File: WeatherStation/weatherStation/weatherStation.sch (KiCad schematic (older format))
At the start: 34 parts, among them J1 RJ12, J3 AVR-ISP-6, J4 USB_B_Micro, SW1 SW_Push, U1 ATmega328P-AU, U2 ATtiny45V-10PU, U3 BME280, U4 FDW254p, U5 FT230XS, U6 MB85RC64, U7 DS3231_Breakout, Y1 Crystal

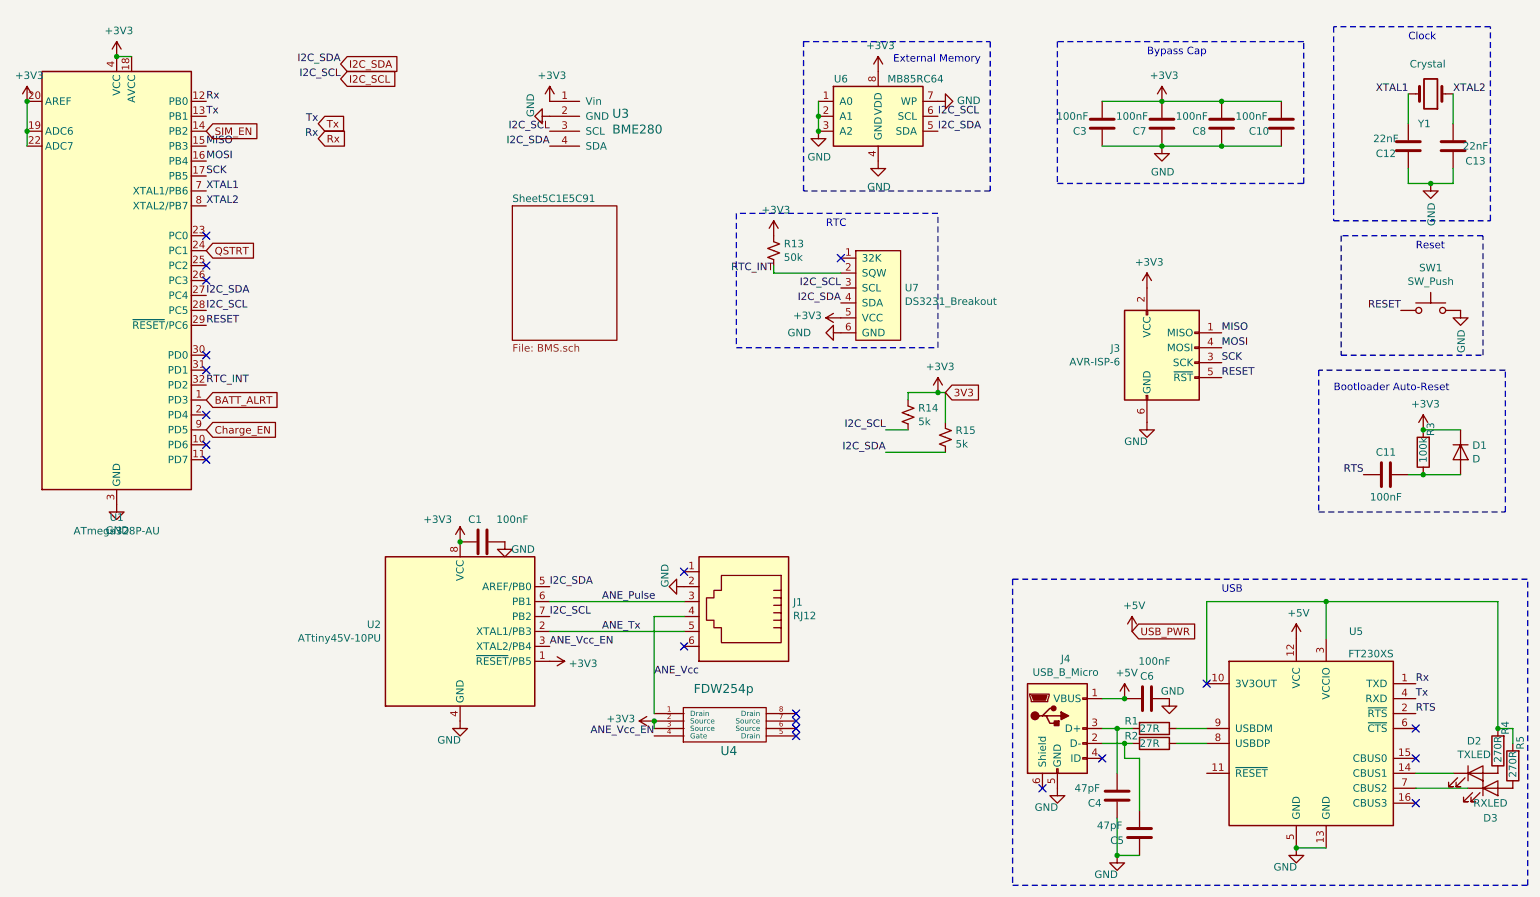
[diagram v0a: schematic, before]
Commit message: commit before more
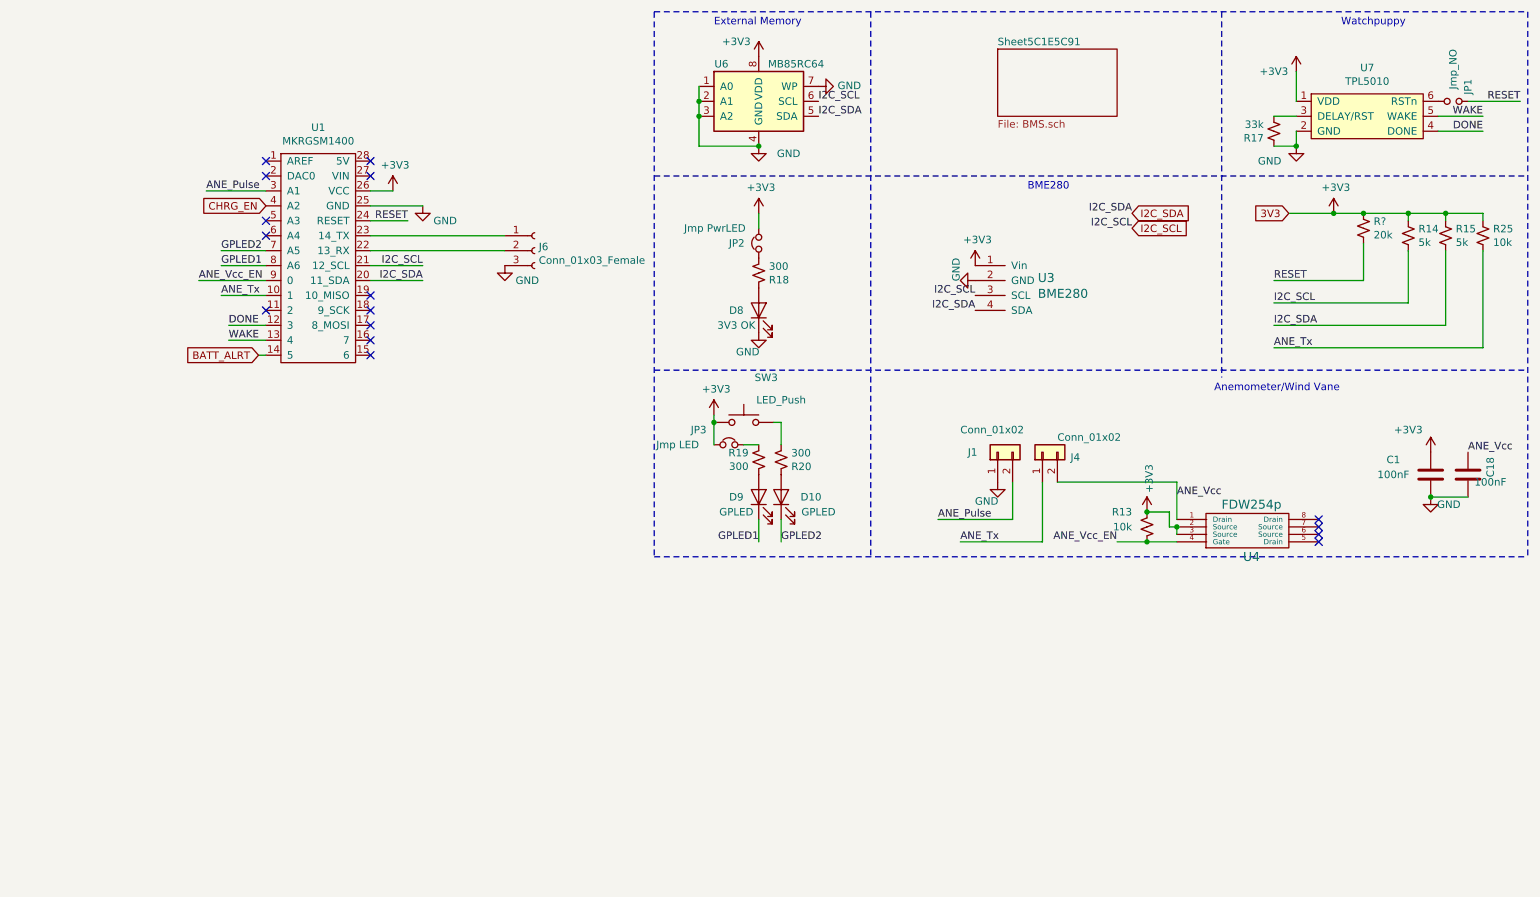
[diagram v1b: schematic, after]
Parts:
- removed C10, C11, C3, C6, C7, C8: 100nF, Capacitor_SMD:C_0805_2012Metric, symbol Device:C
- removed C12, C13: 22nF, Capacitor_SMD:C_0805_2012Metric, symbol Device:C
- removed C4, C5: 47pF, Capacitor_SMD:C_0805_2012Metric, symbol Device:C
- removed D1: D, Diode_SMD:D_SOD-323, symbol Device:D
- removed D2: TXLED, LED_SMD:LED_0805_2012Metric, symbol Device:LED
- removed D3: RXLED, LED_SMD:LED_0805_2012Metric, symbol Device:LED
- removed J1: RJ12, Connector_RJ:RJ12_Amphenol_54601, symbol Connector:RJ12
- removed J3: AVR-ISP-6, Connector_PinHeader_2.54mm:PinHeader_2x03_P2.54mm_Vertical, symbol Connector:AVR-ISP-6
- removed J4: USB_B_Micro, Connector_USB:USB_Micro-B_Amphenol_10103594-0001LF_Horizontal, symbol Connector:USB_B_Micro
- removed R1, R2: 27R, Resistor_SMD:R_0603_1608Metric_Pad1.05x0.95mm_HandSolder, symbol Device:R
- removed R3: 100k, Resistor_SMD:R_0603_1608Metric_Pad1.05x0.95mm_HandSolder, symbol Device:R
- removed R4, R5: 270R, Resistor_SMD:R_0805_2012Metric, symbol Device:R
- removed SW1: SW_Push, EbayParts:Tact_SMD_Switch, symbol Switch:SW_Push
- removed U1: ATmega328P-AU, Package_QFP:TQFP-32_7x7mm_P0.8mm, symbol MCU_Microchip_ATmega:ATmega328P-AU
- removed U2: ATtiny45V-10PU, Package_DIP:DIP-8_W7.62mm_Socket, symbol MCU_Microchip_ATtiny:ATtiny45V-10PU
- removed U5: FT230XS, Package_SO:SSOP-16_3.9x4.9mm_P0.635mm, symbol Interface_USB:FT230XS
- removed U7: DS3231_Breakout, Connector_PinHeader_2.54mm:PinHeader_1x06_P2.54mm_Vertical, symbol CustomComponents:DS3231_Breakout
- removed Y1: Crystal, Crystal:Crystal_HC49-U_Vertical, symbol Device:Crystal
- added C18: 100nF, Capacitor_SMD:C_0805_2012Metric, symbol Device:C
- added D10, D9: GPLED, LED_SMD:LED_0805_2012Metric, symbol Device:LED
- added D8: 3V3 OK, LED_SMD:LED_0805_2012Metric, symbol Device:LED
- added J1, J4: Conn_01x02, Connector_JST:JST_EH_B02B-EH-A_1x02_P2.50mm_Vertical, symbol Connector_Generic:Conn_01x02
- added J6: Conn_01x03_Female, Connector_PinHeader_2.54mm:PinHeader_1x03_P2.54mm_Vertical, symbol Connector:Conn_01x03_Female
- added JP1: Jmp_NO, Jumpers:SMT-JUMPER_2_NO_NO-SILK, symbol Device:Jumper_NO_Small
- added JP2: Jmp PwrLED, Jumpers:SMT-JUMPER_2_NO_NO-SILK, symbol Device:Jumper_NC_Small
- added JP3: Jmp LED, Jumpers:SMT-JUMPER_2_NO_NO-SILK, symbol Device:Jumper_NC_Small
- added R17: 33k, Resistor_SMD:R_0603_1608Metric, symbol Device:R_Small_US
- added R18, R19, R20: 300, Resistor_SMD:R_0603_1608Metric, symbol Device:R_Small_US
- added R25: 10k, Resistor_SMD:R_0603_1608Metric, symbol Device:R_Small_US
- added R?: 20k, Resistor_SMD:R_0603_1608Metric, symbol Device:R_Small_US
- added SW3: LED_Push, EbayParts:Tact_SMD_Switch, symbol Switch:SW_Push
- added U1: MKRGSM1400, CustomFP:MKRGSM1400, symbol CustomComponents:MKRGSM1400
- added U7: TPL5010, Package_TO_SOT_SMD:SOT-23-6, symbol CustomComponents:TPL5010
- R13: value 50k -> 10k
- U3: footprint CustomFP:PinHeader_1x04_P2.54mm_Horizontal -> Connector_JST:JST_EH_B04B-EH-A_1x04_P2.50mm_Vertical
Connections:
- net RTC_INT is gone; now on net ANE_Vcc_EN: R13.2
- net +3V3: now also JP2.2, JP3.1, R25.1, R?.1, SW3.1, U1.26 (VCC), U7.1 (VDD)
- net ANE_Pulse: now also J1.2 (Pin_2), U1.3 (A1)
- net ANE_Tx: now also J4.1 (Pin_1), R25.2, U1.10 (1)
- net ANE_Vcc: now also C18.2, J4.2 (Pin_2)
- net ANE_Vcc_EN: now also U1.9 (0)
- net BATT_ALRT: now also U1.14 (5)
- net GND: now also C18.1, D8.1 (K), J1.1 (Pin_1), J6.3 (Pin_3), R17.1, U1.25 (GND), U7.2 (GND)
- net I2C_SCL: now also U1.21 (12_SCL)
- net I2C_SDA: now also U1.20 (11_SDA)
- net RESET: now also JP1.2, R?.2, U1.24 (RESET)
- new net: D8.2 (A), R18.1
- new net: JP2.1, R18.2
- new net: JP3.2, R19.1
- new net: D9.2 (A), R19.2
- new net: D10.2 (A), R20.1
- new net: R20.2, SW3.2
- new net: R17.2, U7.3 (DELAY/RST)
- new net: JP1.1, U7.6 (RSTn)
- new net: J6.2 (Pin_2), U1.22 (13_RX)
- new net: J6.1 (Pin_1), U1.23 (14_TX)
- new net CHRG_EN: U1.4 (A2)
- new net DONE: U1.12 (3), U7.4 (DONE)
- new net GPLED1: D9.1 (K), U1.8 (A6)
- new net GPLED2: D10.1 (K), U1.7 (A5)
- new net WAKE: U1.13 (4), U7.5 (WAKE)
- no-connect marks 21 -> 16
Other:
- note added: "Anemometer/Wind Vane"
- note added: "BME280"
- note added: "Watchpuppy"
- note removed: "Bootloader Auto-Reset"
- note removed: "Bypass Cap"
- note removed: "Clock"
- note removed: "RTC"
- note removed: "Reset"
- note removed: "USB"
- moved on the sheet: C1, R14, R15, U3, U4, U6
